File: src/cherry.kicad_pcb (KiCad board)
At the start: 2 copper layers, 61.2 x 26.1 mm, 66 parts, among them J1 USB4085-GF-A, J2 PinHeader_2x24, J3 PinHeader_1x06, J4 PinHeader_1x06, J5 PinHeader_1x06, SW1 RESET, SW2 USER, U1 FT2232HQ, U2 ICE40LP8K-CM81, U3 W25Q32JVSSIQ, U4 TPS62A02, U5 TPS62A02, X1 ASE-12.000MHZ-LC-T

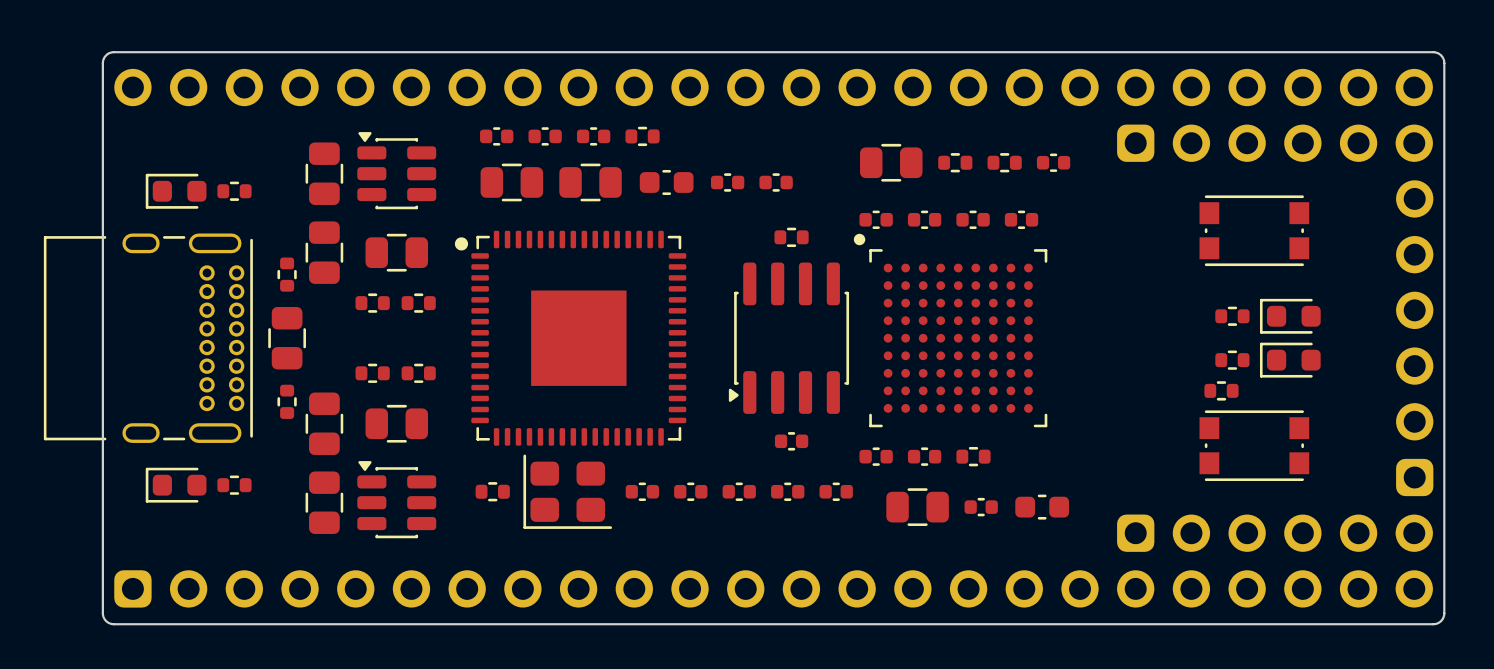
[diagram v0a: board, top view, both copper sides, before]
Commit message: wip
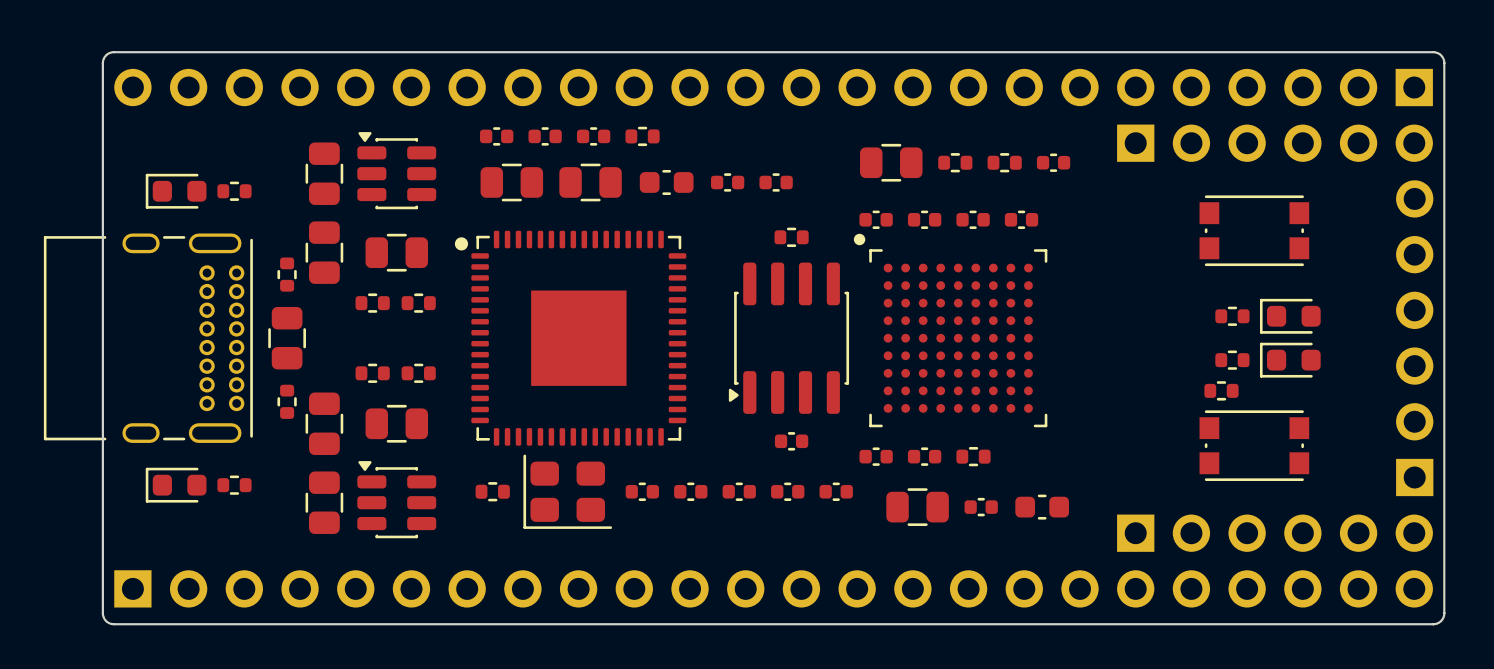
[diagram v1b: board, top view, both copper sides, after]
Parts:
- added J6: PinHeader_1x24, Cherry:PinHeader_1x24_P2.54mm, B.Cu at (159.8, 79.1)
- J2: value PinHeader_2x24 -> PinHeader_1x24; footprint Cherry:PinHeader_2x24_P2.54mm_Rows22.86mm -> Cherry:PinHeader_1x24_P2.54mm; moved to B.Cu
- J3, J4, J5: moved to B.Cu
- R10: value 10k -> 1k
- moved J2 31.4 mm to (101.4, 101.9), turned to -90 degrees
- moved J5 18.9 mm to (147.1, 81.6), turned to -90 degrees
- moved J4 16.5 mm to (159.8, 96.8)
- moved J3 15.5 mm to (147.1, 99.4), turned to -90 degrees
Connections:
- net /GPIO_19 renamed /GPIO_32
- net /GPIO_20 renamed /GPIO_31
- net /GPIO_21 renamed /GPIO_30
- net /GPIO_22 renamed /GPIO_29
- U2 pad A2: /GPIO_27 -> /GPIO_23
- U2 pad A4: /GPIO_23 -> /GPIO_27
- U2 pad A7: /GPIO_18 -> /GPIO_33
- U2 pad A8: /GPIO_16 -> /GPIO_35
- U2 pad B1: /GPIO_0 -> /GPIO_4
- U2 pad B2: /GPIO_2 -> /GPIO_6
- U2 pad B3: /GPIO_26 -> /GPIO_24
- U2 pad B4: /GPIO_24 -> /GPIO_26
- U2 pad B8: /GPIO_17 -> /GPIO_34
- U2 pad C1: /GPIO_1 -> /GPIO_5
- U2 pad C2: /GPIO_3 -> /GPIO_7
- U2 pad C9: /GPIO_9 -> /GPIO_13
- U2 pad D1: /GPIO_4 -> /GPIO_8
- U2 pad D2: /GPIO_5 -> /GPIO_9
- U2 pad D9: /GPIO_8 -> /GPIO_12
- U2 pad E1: /GPIO_6 -> /GPIO_10
- U2 pad E2: /GPIO_7 -> /GPIO_11
- U2 pad F1: /GPIO_10 -> /GPIO_14
- U2 pad G9: /GPIO_11 -> /GPIO_15
- U2 pad H1: /GPIO_12 -> /GPIO_16
- U2 pad J1: /GPIO_13 -> /GPIO_17
- U2 pad J2: /GPIO_14 -> /GPIO_18
- U2 pad J3: /GPIO_15 -> /GPIO_36

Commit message: passive
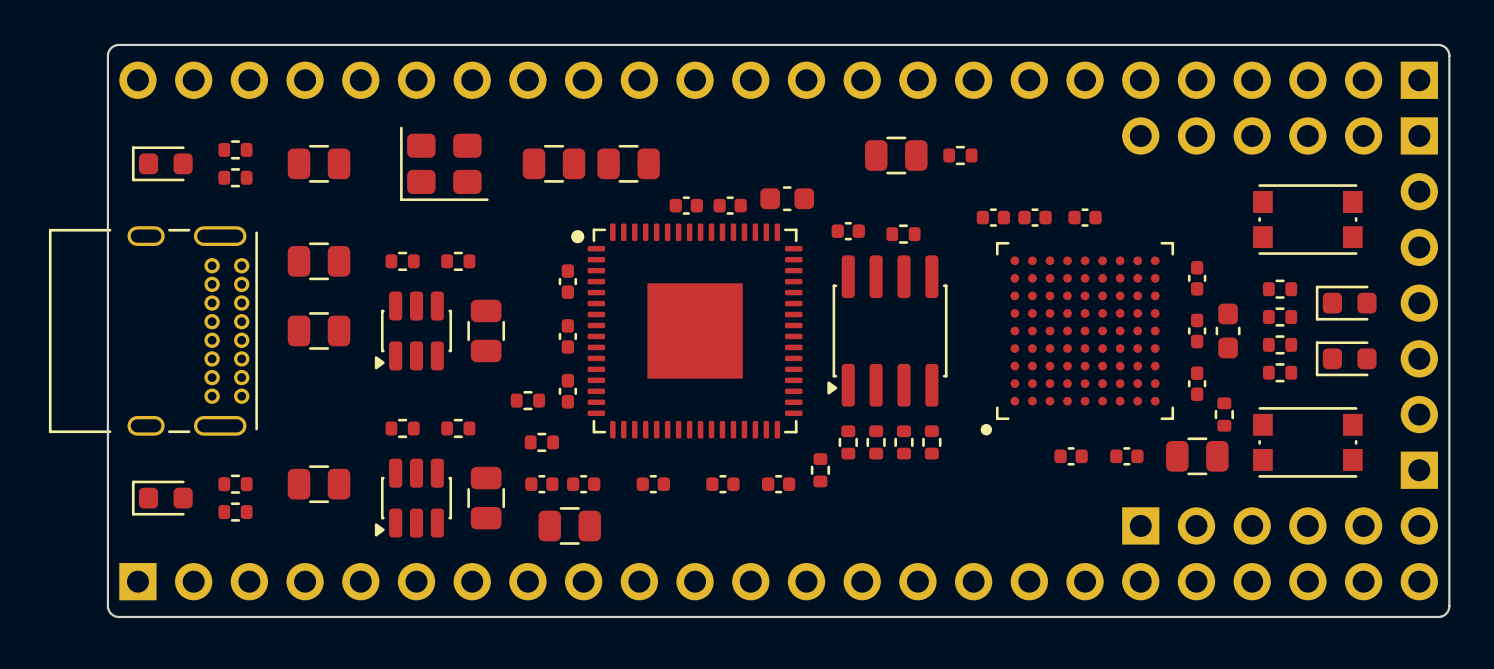
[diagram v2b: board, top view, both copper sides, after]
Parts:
- added R18: 470, Cherry:R_0402_1005Metric, F.Cu at (134.0, 95.2)
- added R19: 470, Cherry:R_0402_1005Metric, F.Cu at (135.3, 95.2)
- added R20: 470, Cherry:R_0402_1005Metric, F.Cu at (136.5, 95.2)
- added R21: 470, Cherry:R_0402_1005Metric, F.Cu at (137.8, 95.2)
- added R22: 1k, Cherry:R_0402_1005Metric, F.Cu at (132.7, 96.5)
- moved C11 16.1 mm to (125.1, 97.2)
- moved X1 16.0 mm to (115.6, 82.5)
- moved C20 15.7 mm to (146.7, 95.9)
- moved C9 14.7 mm to (126.6, 84.5)
- moved R8 14.7 mm to (120.0, 95.2)
- moved C21 14.5 mm to (149.9, 92.6), turned to 90 degrees
- moved R9 13.8 mm to (153.7, 88.3)
- moved C18 13.1 mm to (144.8, 85.0)
- moved C19 13.0 mm to (149.9, 95.9)
- moved J5 12.9 mm to (160.0, 81.3), turned to 90 degrees
- moved C26 12.7 mm to (149.9, 90.2), turned to 90 degrees
- moved C4 12.1 mm to (121.3, 99.1), turned to 0 degrees
- moved C14 11.8 mm to (121.2, 90.4), turned to 90 degrees
- moved C27 11.7 mm to (151.3, 90.2), turned to 90 degrees
- moved C10 11.7 mm to (121.2, 92.9), turned to 90 degrees
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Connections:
- D1 pad 1: Net-(D1-A) -> GND
- D1 pad 2: +3V3 -> Net-(D1-A)
- D2 pad 1: /CDONE -> GND
- J2 pad 1: (no net) -> +5V
- J2 pad 10: (no net) -> /GPIO_4
- J2 pad 11: (no net) -> /GPIO_5
- J2 pad 12: (no net) -> /GPIO_6
- J2 pad 13: (no net) -> /GPIO_7
- J2 pad 14: (no net) -> /GPIO_8
- J2 pad 15: (no net) -> /GPIO_9
- J2 pad 16: (no net) -> /GPIO_10
- J2 pad 17: (no net) -> /GPIO_11
- J2 pad 18: (no net) -> /GPIO_12
- J2 pad 19: (no net) -> /GPIO_13
- J2 pad 2: (no net) -> +3V3
- J2 pad 20: (no net) -> /GPIO_14
- J2 pad 21: (no net) -> /GPIO_15
- J2 pad 22: (no net) -> /GPIO_16
- J2 pad 23: (no net) -> /GPIO_17
- J2 pad 24: (no net) -> /GPIO_18
- J2 pad 3: (no net) -> GND
- J2 pad 4: (no net) -> GND
- J2 pad 5: (no net) -> GND
- J2 pad 6: (no net) -> /CRESET_B
- J2 pad 7: (no net) -> /GPIO_1
- J2 pad 8: (no net) -> /GPIO_2
- J2 pad 9: (no net) -> /GPIO_3
- J3 pad 1: (no net) -> /GPIO_37
- J3 pad 2: (no net) -> /GPIO_38
- J3 pad 3: (no net) -> /GPIO_39
- J3 pad 4: (no net) -> /GPIO_40
- J3 pad 5: (no net) -> /GPIO_41
- J3 pad 6: (no net) -> /GPIO_42
- J4 pad 1: (no net) -> /GPIO_43
- J4 pad 2: (no net) -> /GPIO_44
- J4 pad 3: (no net) -> /GPIO_45
- J4 pad 4: (no net) -> /GPIO_46
- J4 pad 5: (no net) -> /GPIO_47
- J4 pad 6: (no net) -> /GPIO_48
- J5 pad 1: (no net) -> /GPIO_49
- J5 pad 2: (no net) -> /GPIO_50
- J5 pad 3: (no net) -> /GPIO_51
- J5 pad 4: (no net) -> /GPIO_52
- J5 pad 5: (no net) -> /GPIO_53
- J5 pad 6: (no net) -> GND
- J6 pad 1: (no net) -> /GPIO_19
- J6 pad 10: (no net) -> /GPIO_28
- J6 pad 11: (no net) -> /GPIO_29
- J6 pad 12: (no net) -> /GPIO_30
- J6 pad 13: (no net) -> /GPIO_31
- J6 pad 14: (no net) -> /GPIO_32
- J6 pad 15: (no net) -> /GPIO_33
- J6 pad 16: (no net) -> /GPIO_34
- J6 pad 17: (no net) -> /GPIO_35
- J6 pad 18: (no net) -> /GPIO_36
- J6 pad 19: (no net) -> GND
- J6 pad 2: (no net) -> /GPIO_20
- J6 pad 20: (no net) -> GND
- J6 pad 21: (no net) -> GND
- J6 pad 22: (no net) -> GND
- J6 pad 23: (no net) -> +3V3
- J6 pad 24: (no net) -> +5V
- J6 pad 3: (no net) -> /GPIO_21
- J6 pad 4: (no net) -> /GPIO_22
- J6 pad 5: (no net) -> /GPIO_23
- J6 pad 6: (no net) -> /GPIO_24
- J6 pad 7: (no net) -> /GPIO_25
- J6 pad 8: (no net) -> /GPIO_26
- J6 pad 9: (no net) -> /GPIO_27
- R14 pad 1: Net-(D1-A) -> +3V3
- R14 pad 2: GND -> Net-(D1-A)
- R15 pad 1: +3V3 -> /CDONE
- R8 pad 2: /FT_RESET -> Net-(U1-~{RESET})
- U1 pad 1: (no net) -> GND
- U1 pad 10: (no net) -> GND
- U1 pad 11: (no net) -> GND
- U1 pad 12: (no net) -> /VCORE
- U1 pad 13: (no net) -> GND
- U1 pad 14: (no net) -> Net-(U1-~{RESET})
- U1 pad 15: (no net) -> GND
- U1 pad 16: (no net) -> /FT_SCK
- U1 pad 17: (no net) -> /FT_MOSI
- U1 pad 18: (no net) -> /FT_MISO
- U1 pad 19: (no net) -> unconnected-(U1-ADBUS3-Pad19)
- U1 pad 2: (no net) -> /CLK_12M
- U1 pad 20: (no net) -> +3V3
- U1 pad 21: (no net) -> /FT_SS
- U1 pad 22: (no net) -> unconnected-(U1-ADBUS5-Pad22)
- U1 pad 23: (no net) -> /CDONE
- U1 pad 24: (no net) -> /FT_CRESET
- U1 pad 25: (no net) -> GND
- U1 pad 26: (no net) -> unconnected-(U1-ACBUS0-Pad26)
- U1 pad 27: (no net) -> unconnected-(U1-ACBUS1-Pad27)
- U1 pad 28: (no net) -> unconnected-(U1-ACBUS2-Pad28)
- U1 pad 29: (no net) -> unconnected-(U1-ACBUS3-Pad29)
- U1 pad 3: (no net) -> unconnected-(U1-OSCO-Pad3)
- U1 pad 30: (no net) -> unconnected-(U1-ACBUS4-Pad30)
- U1 pad 31: (no net) -> +3V3
- U1 pad 32: (no net) -> unconnected-(U1-ACBUS5-Pad32)
- U1 pad 33: (no net) -> unconnected-(U1-ACBUS6-Pad33)
- U1 pad 34: (no net) -> unconnected-(U1-ACBUS7-Pad34)
- U1 pad 35: (no net) -> GND
- U1 pad 36: (no net) -> unconnected-(U1-~{SUSPEND}-Pad36)
- U1 pad 37: (no net) -> /VCORE
- U1 pad 38: (no net) -> /UART_TX
- U1 pad 39: (no net) -> /UART_RX
- U1 pad 4: (no net) -> /+3V3A
- U1 pad 40: (no net) -> unconnected-(U1-BDBUS2-Pad40)
- U1 pad 41: (no net) -> unconnected-(U1-BDBUS3-Pad41)
- U1 pad 42: (no net) -> +3V3
- U1 pad 43: (no net) -> unconnected-(U1-BDBUS4-Pad43)
- U1 pad 44: (no net) -> unconnected-(U1-BDBUS5-Pad44)
- U1 pad 45: (no net) -> unconnected-(U1-BDBUS6-Pad45)
- U1 pad 46: (no net) -> unconnected-(U1-BDBUS7-Pad46)
- U1 pad 47: (no net) -> GND
- U1 pad 48: (no net) -> unconnected-(U1-BCBUS0-Pad48)
- U1 pad 49: (no net) -> /VCORE
- U1 pad 5: (no net) -> GND
- U1 pad 50: (no net) -> +3V3
- U1 pad 51: (no net) -> GND
- U1 pad 52: (no net) -> unconnected-(U1-BCBUS1-Pad52)
- U1 pad 53: (no net) -> unconnected-(U1-BCBUS2-Pad53)
- U1 pad 54: (no net) -> unconnected-(U1-BCBUS3-Pad54)
- U1 pad 55: (no net) -> unconnected-(U1-BCBUS4-Pad55)
- U1 pad 56: (no net) -> +3V3
- U1 pad 57: (no net) -> unconnected-(U1-BCBUS5-Pad57)
- U1 pad 58: (no net) -> unconnected-(U1-BCBUS6-Pad58)
- U1 pad 59: (no net) -> unconnected-(U1-BCBUS7-Pad59)
- U1 pad 6: (no net) -> Net-(U1-REF)
- U1 pad 60: (no net) -> unconnected-(U1-~{PWREN}-Pad60)
- U1 pad 61: (no net) -> unconnected-(U1-EEDATA-Pad61)
- U1 pad 62: (no net) -> unconnected-(U1-EECLK-Pad62)
- U1 pad 63: (no net) -> unconnected-(U1-EECS-Pad63)
- U1 pad 64: (no net) -> /VCORE
- U1 pad 65: (no net) -> GND
- U1 pad 7: (no net) -> /USB_DM
- U1 pad 8: (no net) -> /USB_DP
- U1 pad 9: (no net) -> /+3V3A
- U2 pad A1: unconnected-(U2-IOT_224-PadA1) -> /GPIO_34
- U2 pad A2: /GPIO_23 -> /GPIO_33
- U2 pad A3: /GPIO_25 -> /GPIO_31
- U2 pad A6: /GPIO_31 -> /GPIO_24
- U2 pad A7: /GPIO_33 -> /GPIO_21
- U2 pad A8: /GPIO_35 -> /GPIO_20
- U2 pad A9: unconnected-(U2-IOR_116-PadA9) -> /GPIO_46
- U2 pad B1: /GPIO_4 -> /GPIO_3
- U2 pad B2: /GPIO_6 -> /GPIO_2
- U2 pad B3: /GPIO_24 -> /GPIO_32
- U2 pad B4: /GPIO_26 -> /GPIO_28
- U2 pad B5: /GPIO_29 -> /GPIO_25
- U2 pad B6: /GPIO_30 -> /GPIO_23
- U2 pad B7: /GPIO_32 -> /GPIO_22
- U2 pad B8: /GPIO_34 -> /GPIO_19
- U2 pad B9: unconnected-(U2-IOR_120-PadB9) -> /GPIO_50
- U2 pad C1: /GPIO_5 -> /GPIO_4
- U2 pad C2: /GPIO_7 -> /GPIO_1
- U2 pad C3: unconnected-(U2-IOL_7B-PadC3) -> /GPIO_6
- U2 pad C4: /CLK_12M -> /BTN
- U2 pad C5: unconnected-(U2-IOT_197_GBIN1-PadC5) -> /GPIO_26
- U2 pad C9: /GPIO_13 -> /GPIO_53
- U2 pad D1: /GPIO_8 -> /GPIO_7
- U2 pad D2: /GPIO_9 -> /GPIO_5
- U2 pad D3: unconnected-(U2-IOL_13B_GBIN7-PadD3) -> /GPIO_10
- U2 pad D5: unconnected-(U2-IOT_212-PadD5) -> /GPIO_29
- U2 pad D6: unconnected-(U2-IOR_115-PadD6) -> /GPIO_45
- U2 pad D7: unconnected-(U2-IOR_117-PadD7) -> /GPIO_47
- U2 pad D8: unconnected-(U2-IOR_141_GBIN2-PadD8) -> /GPIO_52
- U2 pad D9: /GPIO_12 -> /GPIO_49
- U2 pad E1: /GPIO_10 -> /GPIO_8
- U2 pad E2: /GPIO_11 -> /GPIO_9
- U2 pad E3: unconnected-(U2-IOL_14A_GBIN6-PadE3) -> /GPIO_11
- U2 pad E4: unconnected-(U2-IOL_14B-PadE4) -> /GPIO_12
- U2 pad E5: unconnected-(U2-IOT_214-PadE5) -> /GPIO_30
- U2 pad E7: unconnected-(U2-IOR_118-PadE7) -> /GPIO_48
- U2 pad E8: unconnected-(U2-IOR_140_GBIN3-PadE8) -> /GPIO_51
- U2 pad F1: /GPIO_14 -> /GPIO_13
- U2 pad F3: unconnected-(U2-IOL_22B-PadF3) -> /GPIO_14
- U2 pad F8: unconnected-(U2-IOR_113-PadF8) -> /GPIO_43
- U2 pad G1: unconnected-(U2-IOL_24B-PadG1) -> /GPIO_16
- U2 pad G2: unconnected-(U2-IOL_26A-PadG2) -> /GPIO_17
- U2 pad G3: unconnected-(U2-IOL_24A-PadG3) -> /GPIO_15
- U2 pad G4: unconnected-(U2-IOB_81_GBIN5-PadG4) -> /CLK_12M
- U2 pad G5: unconnected-(U2-IOB_103_CBSEL0-PadG5) -> /GPIO_40
- U2 pad G8: unconnected-(U2-IOR_114-PadG8) -> /GPIO_44
- U2 pad G9: /GPIO_15 -> /GPIO_42
- U2 pad H1: /GPIO_16 -> /GPIO_35
- U2 pad H2: unconnected-(U2-IOL_26B-PadH2) -> /GPIO_18
- U2 pad H4: /BTN -> /GPIO_39
- U2 pad H5: unconnected-(U2-IOB_104_CBSEL1-PadH5) -> /GPIO_41
- U2 pad J1: /GPIO_17 -> /GPIO_36
- U2 pad J2: /GPIO_18 -> /GPIO_37
- U2 pad J3: /GPIO_36 -> /GPIO_38
- U2 pad J4: /UART_TX -> /LED0
- U2 pad J8: /LED0 -> /UART_TX
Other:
- board text added: "NextMicon Cherry v1"
- board text removed: "Cherry"
